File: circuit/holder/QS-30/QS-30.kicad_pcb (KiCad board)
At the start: 2 copper layers, 20.8 x 20.6 mm, 2 parts, among them J1 Nixie_Conn_12P

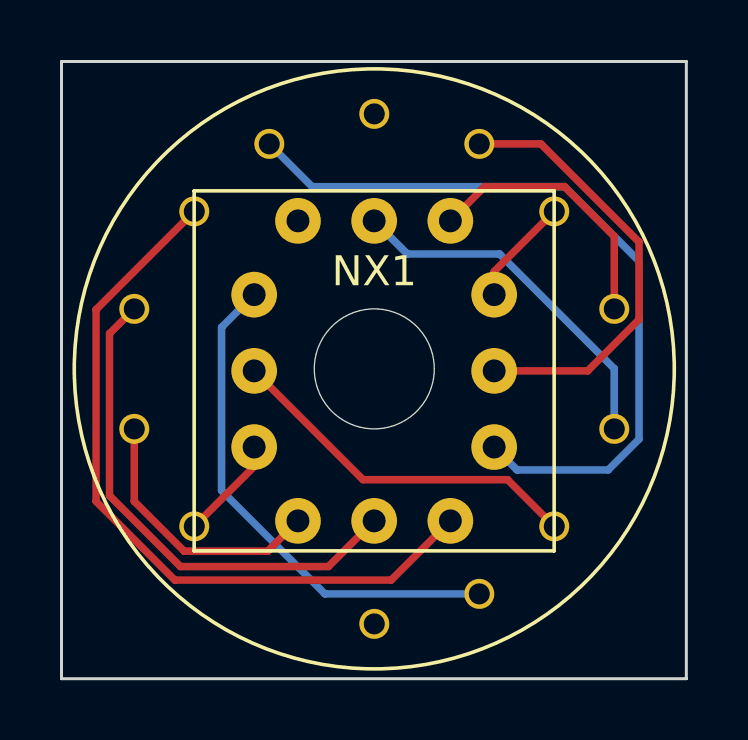
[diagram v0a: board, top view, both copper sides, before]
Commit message: Update schematics
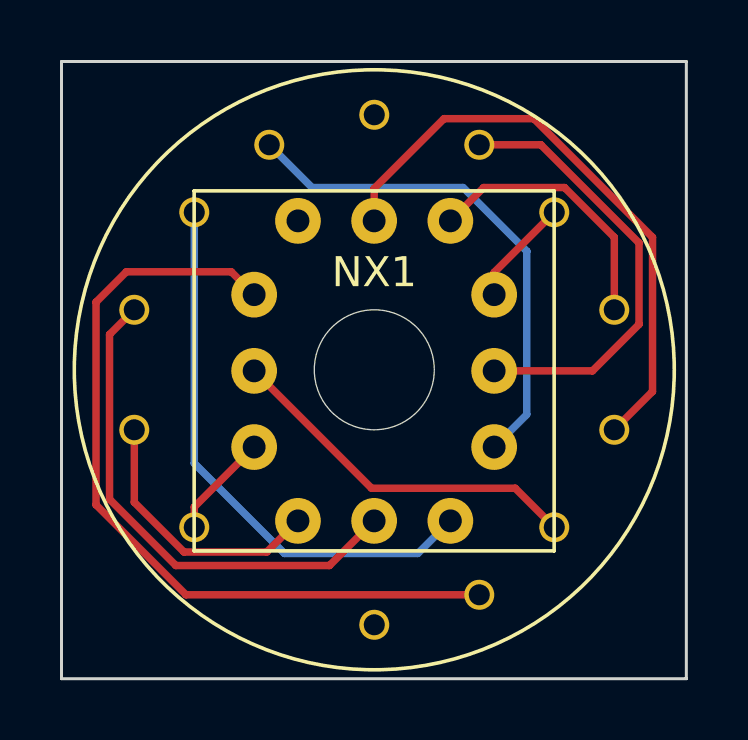
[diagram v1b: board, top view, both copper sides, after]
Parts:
- NX1: value QS27-1 -> QS30-1
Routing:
- net PA: track 17.0 -> 26.8 mm
- net P5: track 25.4 -> 17.0 mm
- net P9: track 12.1 -> 19.9 mm
- net P4: track 24.7 -> 18.6 mm
